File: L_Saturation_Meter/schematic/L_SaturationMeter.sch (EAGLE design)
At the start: 82 parts, among them IC1 LM317, IC4 LM358, SW1 DUR_10X, T1 IRF830, T2 BC847, T3 BC847, T4 BC847, T5 BC847, T6 IRF830, T7 IRF830, X1 I_SENSE_100x, X2 POWER_12V, X3 L_TEST_END, X4 I_SENSE_10x, X5 Synchro, X6 L_TEST_END

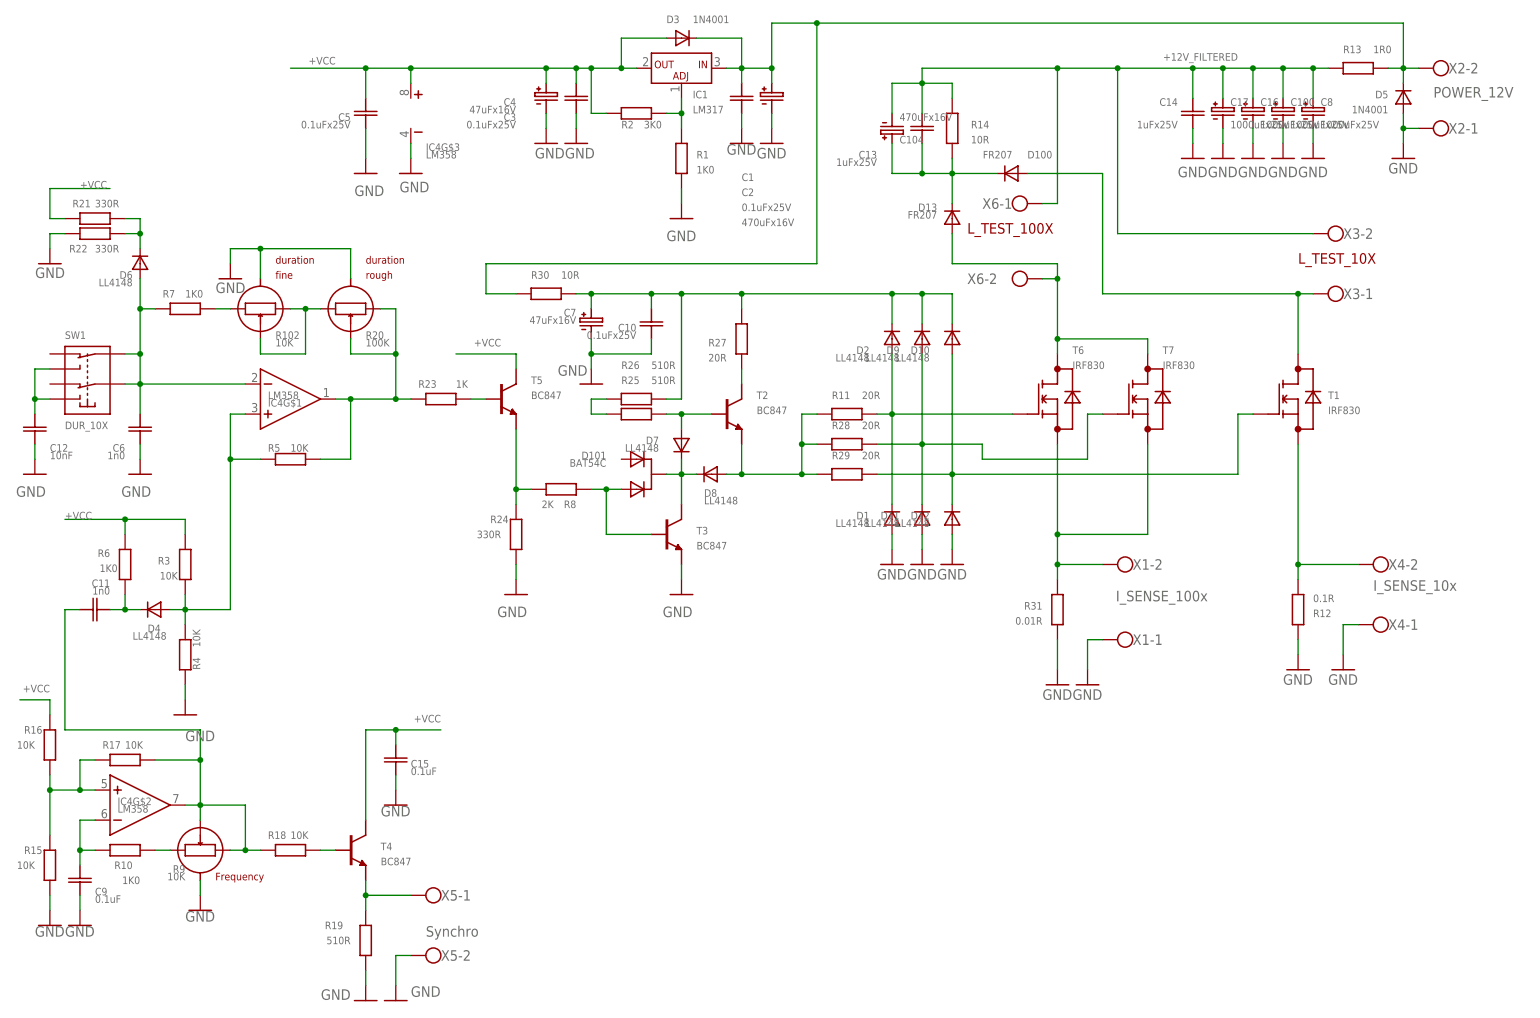
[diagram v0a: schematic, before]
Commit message: L saturation meter. Routing step 1
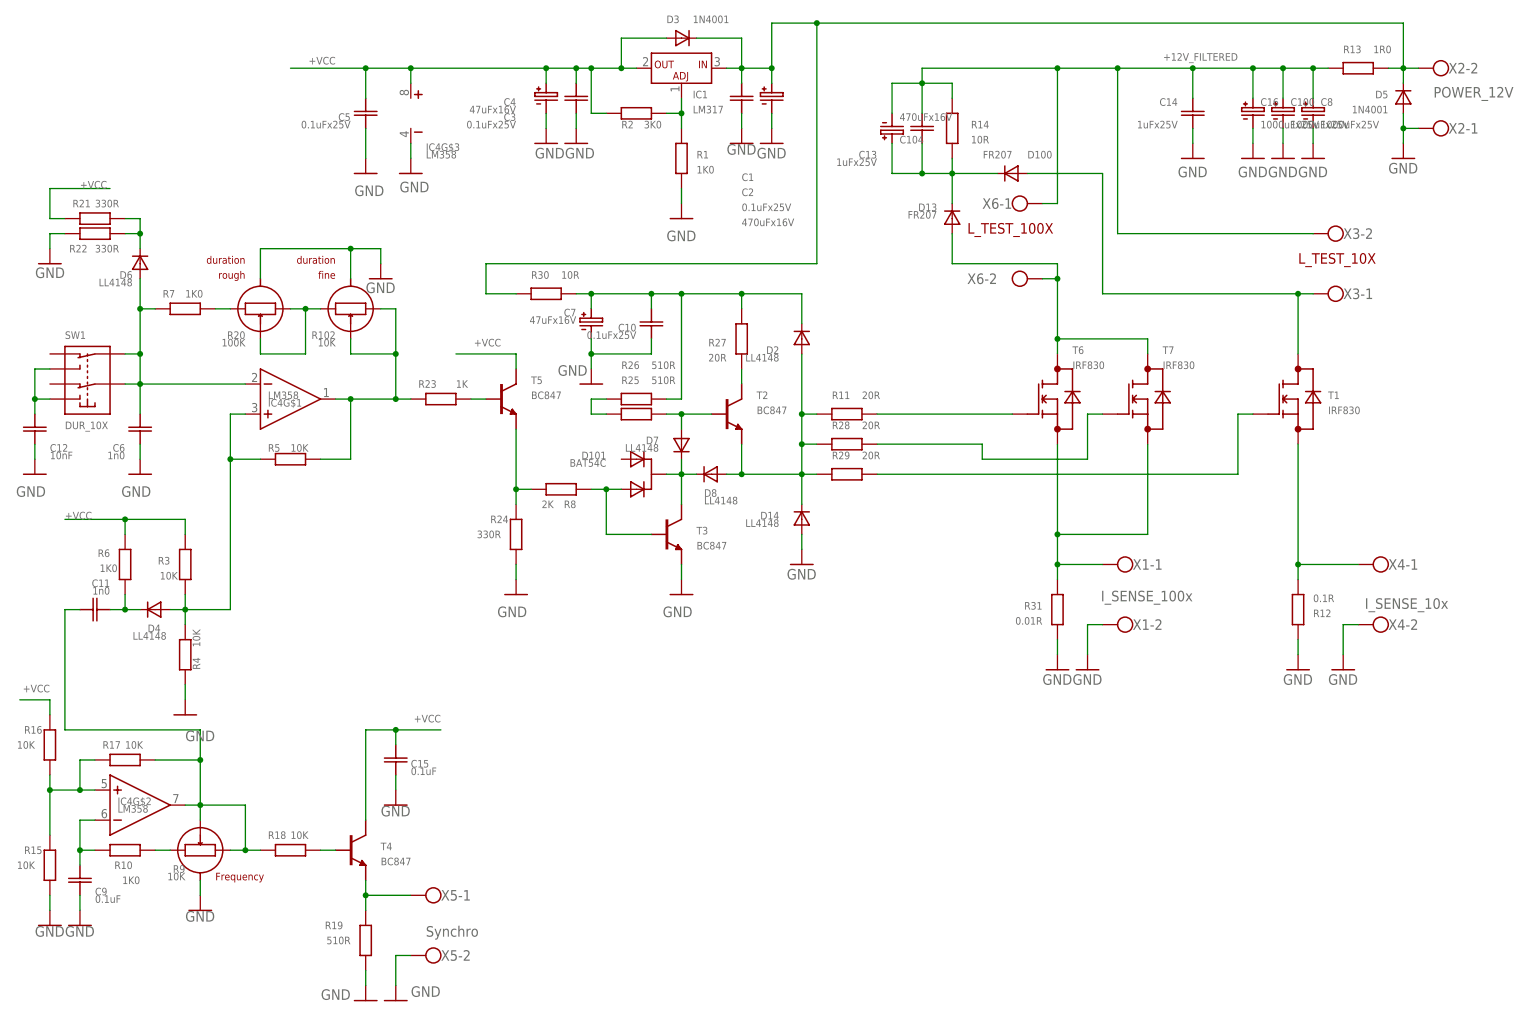
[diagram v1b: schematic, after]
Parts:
- removed C17: 1000uFx25V, __MyCommonLib1:CE10MM
- removed D1, D10, D11, D12, D9: LL4148, __MyCommonLib1:LL4147SOD-80
- added D14: LL4148, __MyCommonLib1:LL4147SOD-80
- D100: device __MyCommonLib1:1N4001DO-41_10MM -> __MyCommonLib1:1N4001DO-41_20MM
- D13: device __MyCommonLib1:1N4001DO-41_10MM -> __MyCommonLib1:1N4001DO-41_5MM
- D3: device __MyCommonLib1:1N4001DO-41_10MM -> __MyCommonLib1:1N4001DO-41_15MM
- D5: device __MyCommonLib1:1N4001DO-41_5MM -> __MyCommonLib1:1N4001DO-41_15MM
- R19, R23: device __MyCommonLib1:RSMD_0805 -> __MyCommonLib1:RSMD_1206_BIG_GAP
- T1, T6, T7: device __MyCommonLib1:IRF830TO-200(HORIZONTAL_SCREW_PAD) -> __MyCommonLib1:IRF830D2PAK
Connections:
- removed net N$17: R102.END_B, R7.PIN0
- new net N$35: R20.END_A, R7.PIN0
- net +12V_FILTERED: no longer C17.PLUS
- net GND: now also D14.ANODE, X1-2.KL, X4-2.KL; no longer C17.MINUS, D1.ANODE, D11.ANODE, D12.ANODE, X1-1.KL, X4-1.KL
- net N$15: now also R20.MIDDLE; no longer R102.MIDDLE
- net N$2: no longer D1.CATHODE, D2.ANODE
- net N$23: now also R102.END_B, R102.MIDDLE; no longer R20.END_A, R20.MIDDLE
- net N$28: no longer D11.CATHODE, D9.ANODE
- net N$3: now also X4-1.KL; no longer X4-2.KL
- net N$30: now also D14.CATHODE, D2.ANODE
- net N$31: no longer D10.ANODE, D12.CATHODE
- net N$32: now also X1-1.KL; no longer X1-2.KL
- net N$33: no longer D10.CATHODE, D9.CATHODE
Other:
- moved on the sheet: D2, R102, R20, X1-1, X1-2, X4-1, X4-2
